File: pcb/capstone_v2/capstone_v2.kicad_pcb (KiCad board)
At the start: 2 copper layers, 19 parts, among them IC1 HSFPAR004A, J10 NCS, J11 NCS, J13 NCS, J14 NCS, J2 VDDA, J3 VDD, J4 VDDIO, J5 GPIO, J6 INT, J7 MISO, J8 MOSI, J9 SCLK

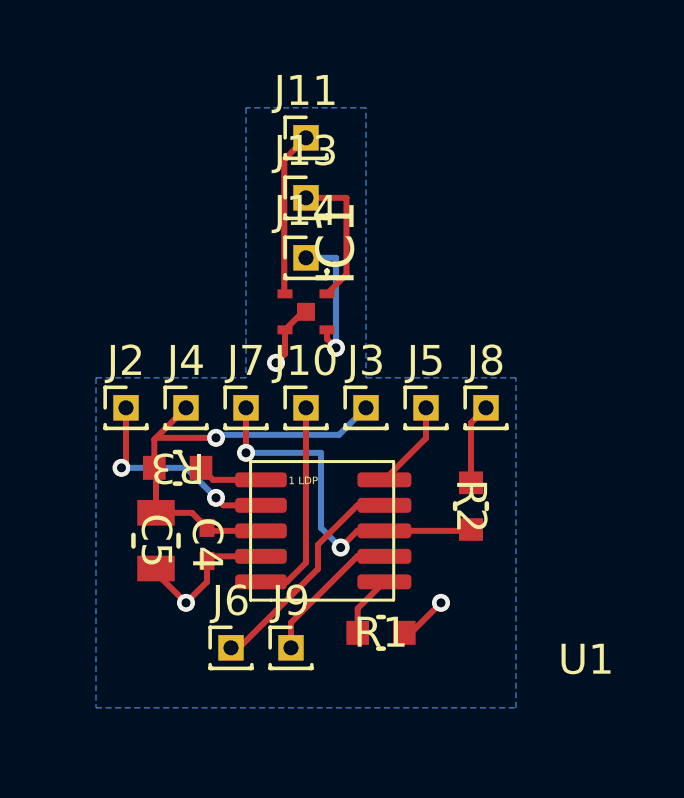
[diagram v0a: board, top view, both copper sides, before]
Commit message: sensor and mcu board nearly complete
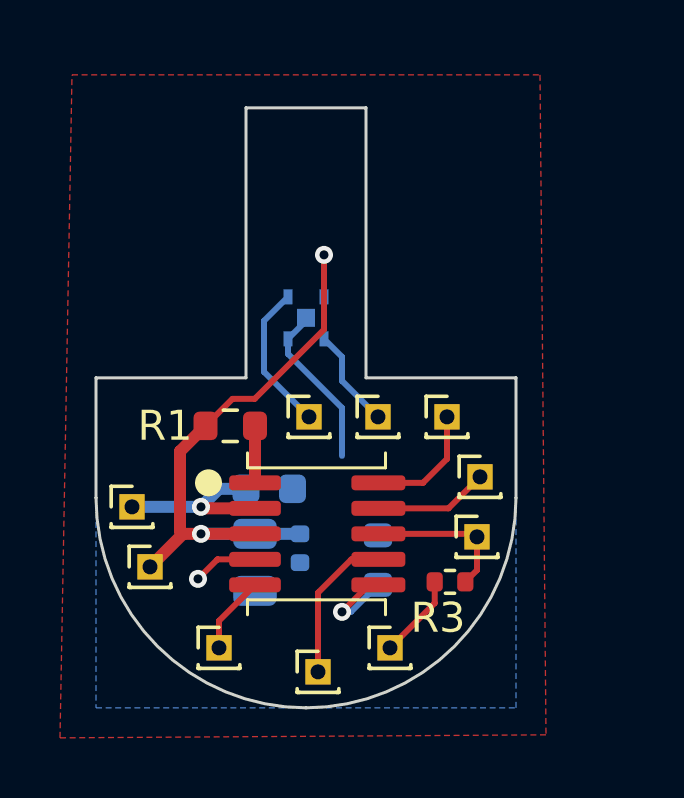
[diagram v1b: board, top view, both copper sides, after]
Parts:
- removed C4: 0.1uF, Library:CAP_CL05_SAM
- removed C5: 10uF, Library:CAP_CL21_SAM
- removed J11, J13, J14: NCS, Connector_PinHeader_1.00mm:PinHeader_1x01_P1.00mm_Vertical
- added C1: 10uF, Capacitor_SMD:C_0805_2012Metric, B.Cu at (96.8, 87.7)
- added C2: 0.1uF, Capacitor_SMD:C_0402_1005Metric, B.Cu at (98.3, 87.2)
- added C3: 1uF, Capacitor_SMD:C_0603_1608Metric, B.Cu at (97.3, 85.2)
- added J1: VDD, Connector_PinHeader_1.00mm:PinHeader_1x01_P1.00mm_Vertical, F.Cu at (93.3, 87.8)
- IC1: footprint Library:HSFPAR004A -> Imported_FP:HSFPAR004A; moved to B.Cu
- J10: value NCS -> FORCE_V1
- J3: value VDD -> NCS
- J4: value VDDIO -> FORCE_V2
- J5: value GPIO -> SCLK
- J6: value INT -> GPIO
- J7: value MISO -> INT
- J8: value MOSI -> MISO
- J9: value SCLK -> MOSI
- R1: value 100k -> 140; footprint Library:RC0603N_PAN -> Resistor_SMD:R_0603_1608Metric
- R2: value 3.3k -> 100k; footprint Library:RC0603N_PAN -> Resistor_SMD:R_0603_1608Metric; moved to B.Cu
- R3: value 140 -> 3.3k; footprint Library:RC0603N_PAN -> Resistor_SMD:R_0402_1005Metric
- U1: value ~ -> PAW3040E1-TKMT; footprint Library:Optical_Sensor -> Imported_FP:PAW3040E1-TKMT
- moved J6 10.5 mm to (103.2, 82.8)
- moved U1 10.1 mm to (98.8, 86.7)
- moved R3 9.84 mm to (103.3, 88.3), turned to 0 degrees
- moved J5 9.51 mm to (98.9, 91.3)
- moved J3 9.38 mm to (95.6, 90.5)
- moved R1 8.54 mm to (96.0, 83.1), turned to 180 degrees
- moved J7 8.13 mm to (104.3, 84.8)
- moved J8 4.31 mm to (104.2, 86.8)
- moved J4 4.11 mm to (98.6, 82.8)
- moved R2 3.58 mm to (100.9, 87.6), turned to 90 degrees
- moved J2 3.31 mm to (92.7, 85.8)
- moved J9 3.30 mm to (101.3, 90.5)
- moved J10 2.42 mm to (100.9, 82.8)
- moved IC1 0.20 mm to (98.5, 79.5), turned to 180 degrees
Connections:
- net Net-(J2-Pin_1) renamed +1.9V
- IC1 pad 1: Net-(IC1-VDD) -> +3.3V
- J10 pad 1: Net-(J10-Pin_1) -> Net-(IC1-V1)
- J4 pad 1: Net-(J3-Pin_1) -> Net-(IC1-V2)
- R1 pad 1: Net-(U1-Reserve) -> Net-(U1-LDP)
- R1 pad 2: GND -> +3.3V
- R2 pad 1: Net-(J8-Pin_1) -> Net-(U1-Reserve)
- R2 pad 2: Net-(J7-Pin_1) -> GND
- R3 pad 1: Net-(U1-LDP) -> Net-(J9-Pin_1)
- R3 pad 2: Net-(J3-Pin_1) -> Net-(J8-Pin_1)
- U1 pad 10: Net-(J5-Pin_1) -> Net-(J6-Pin_1)
- U1 pad 3: Net-(J3-Pin_1) -> +3.3V
- U1 pad 5: Net-(J10-Pin_1) -> Net-(J3-Pin_1)
- U1 pad 7: Net-(J9-Pin_1) -> Net-(J5-Pin_1)
- U1 pad 8: Net-(J7-Pin_1) -> Net-(J8-Pin_1)
- U1 pad 9: Net-(J6-Pin_1) -> Net-(J7-Pin_1)
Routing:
- net +3.3V: track 0.00 -> 20.5 mm, vias 0 -> 2
- net Net-(J3-Pin_1): track 15.1 -> 2.60 mm, vias 1 -> 0
- net Net-(J7-Pin_1): track 12.0 -> 3.82 mm, vias 2 -> 0
- net Net-(J10-Pin_1): track 6.93 -> 0.00 mm
- net Net-(IC1-VDD): track 4.82 -> 0.00 mm
- net Net-(J6-Pin_1): track 7.55 -> 4.02 mm
- net Net-(J8-Pin_1): track 2.71 -> 4.99 mm
- net Net-(IC1-V1): track 5.51 -> 3.35 mm
- net Net-(J5-Pin_1): track 2.97 -> 5.11 mm
- net Net-(J9-Pin_1): track 4.87 -> 2.82 mm
- net GND: track 9.27 -> 7.76 mm, vias 3 -> 1
- net +1.9V: track 7.23 -> 5.87 mm, vias 2 -> 1
- net Net-(U1-Reserve): track 2.07 -> 3.21 mm, vias 0 -> 1
- net Net-(IC1-V2): track 4.72 -> 4.95 mm, vias 1 -> 0
- added copper zone on F.Cu, net GND
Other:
- board outline added: 14 x 20 mm
